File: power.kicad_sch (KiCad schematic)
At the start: 43 parts, among them J3 Battery, J4 Motor, Q1 SiS415DNT, Q2 SiS454DN, Q3 SiS415DNT, Q4 SiS454DN, Q5 SiS415DNT, Q6 SiS454DN, U5 FD6288Q, U6 MAX15062A, U7 INA186

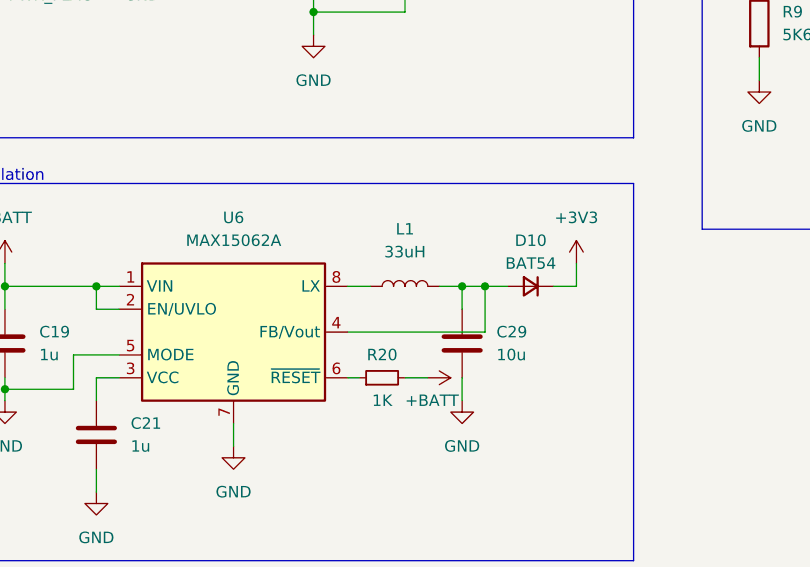
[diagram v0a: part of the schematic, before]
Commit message: finish layout
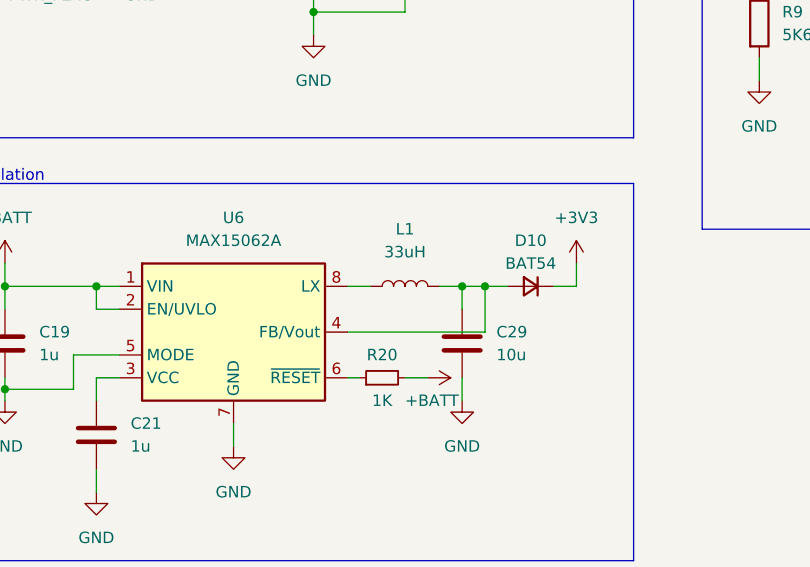
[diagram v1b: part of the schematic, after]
